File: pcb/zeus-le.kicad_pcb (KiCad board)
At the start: 6 copper layers, 50 x 50 mm, 81 parts, among them J1 12402012E212A, J2 S2B-PH-SM4-TB, J3 B5B-PH-K-S, J4 BD125-10-A-0305-0580-L-B, J5 MSD-1-A, J6 B2B-PH-K-S, SW1 EVQPUD02K, U1 NUF2042XV6T1G, U10 D3V3F4U6S-7, U2 RT6160AWSC, U3 KTS1662EUW-TR, U4 BQ25150YFPR, U5 TLV320ADC6120IRTER, U6 WT02C40C-V3, U7 AP21510FM-7, U8 TPD6F003DQDR, U9 LP5810ADSDR

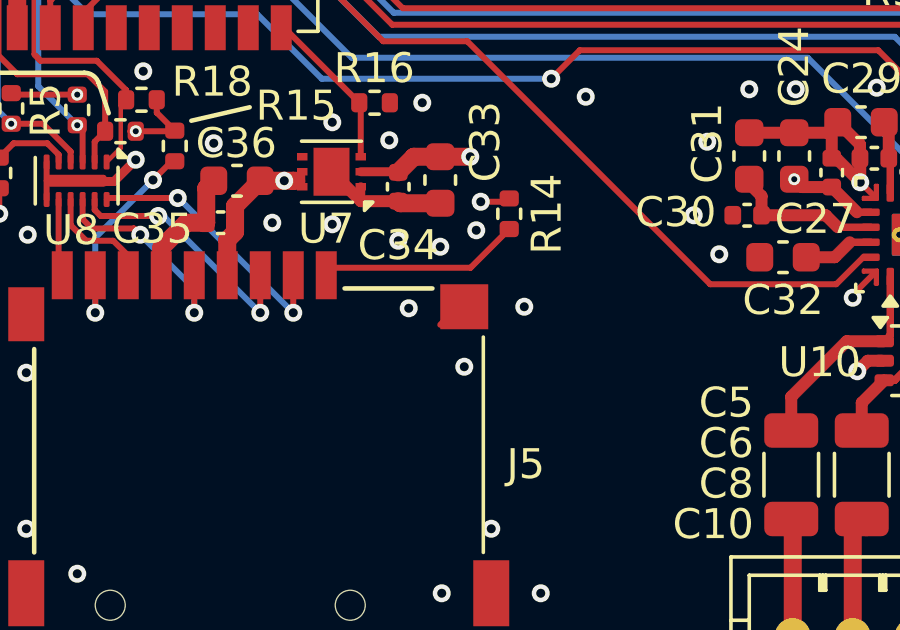
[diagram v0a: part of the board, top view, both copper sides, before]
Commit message: pcb: remove stray trace
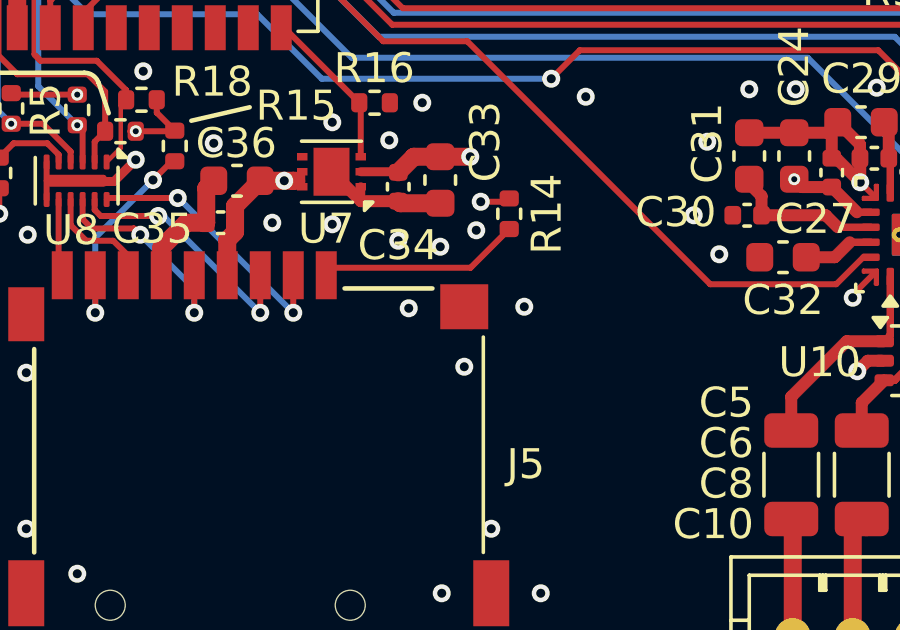
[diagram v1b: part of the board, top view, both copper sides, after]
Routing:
- net GND: track 57.6 -> 56.7 mm
